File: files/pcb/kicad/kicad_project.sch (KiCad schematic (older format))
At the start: 19 parts, among them IC1 ATMEGA328-A, P1 CONN_6, SW1 SW_PUSH, U15 MY_PIN52, U16 MY_PIN52, U17 MY_PIN52, U18 MY_PIN52, X1 12MHz

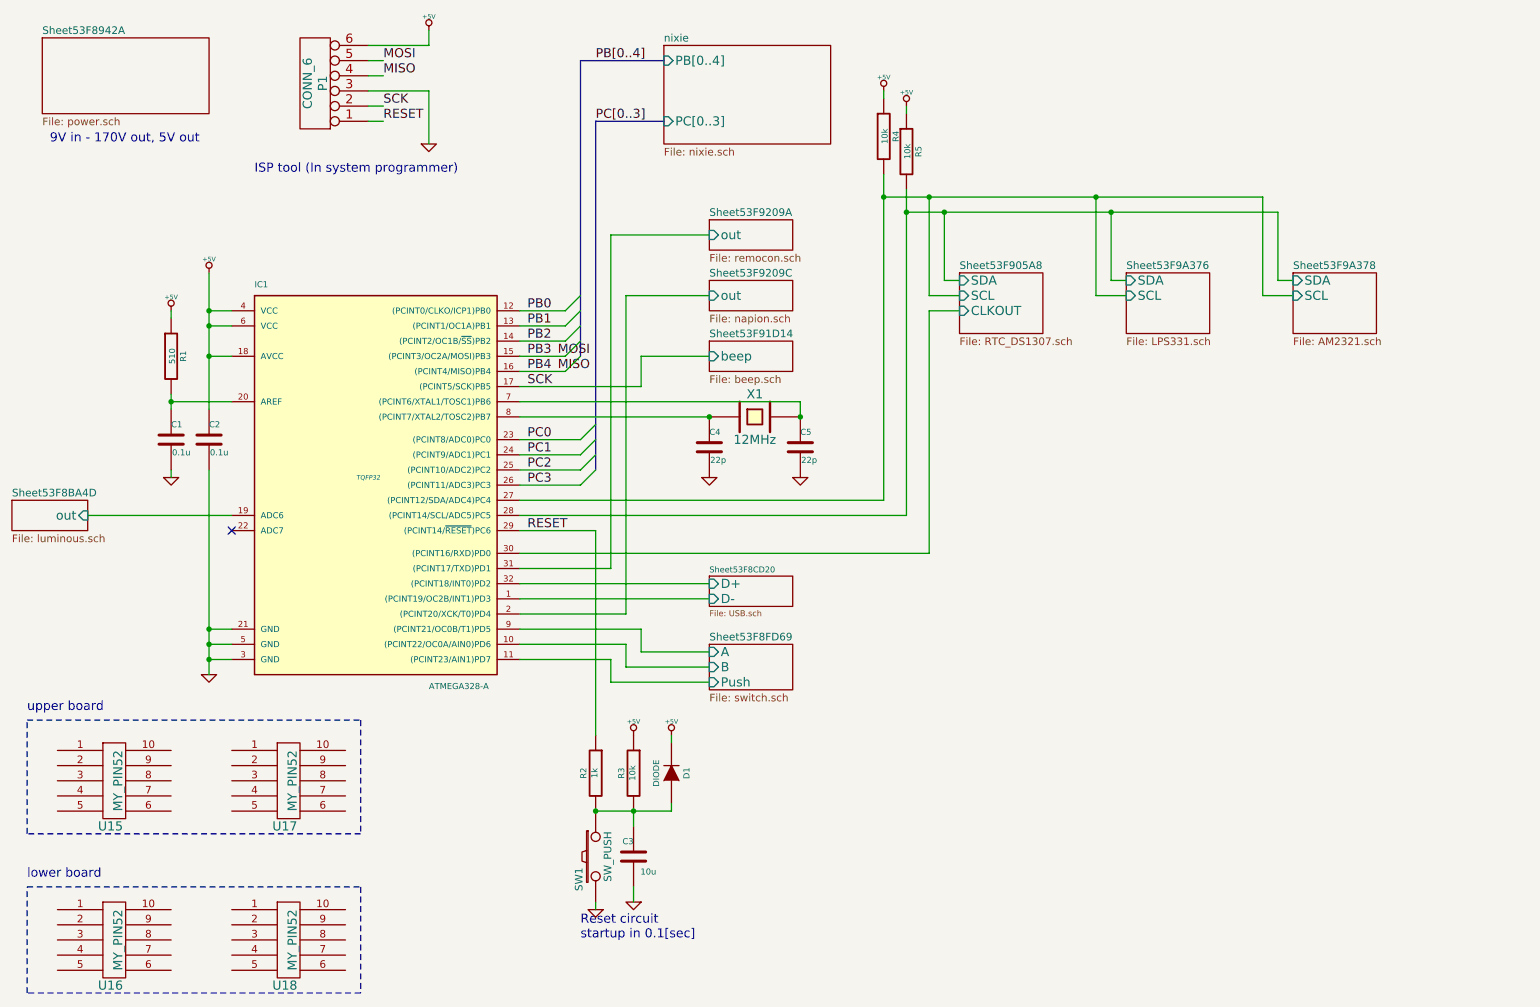
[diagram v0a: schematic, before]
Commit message: PCB
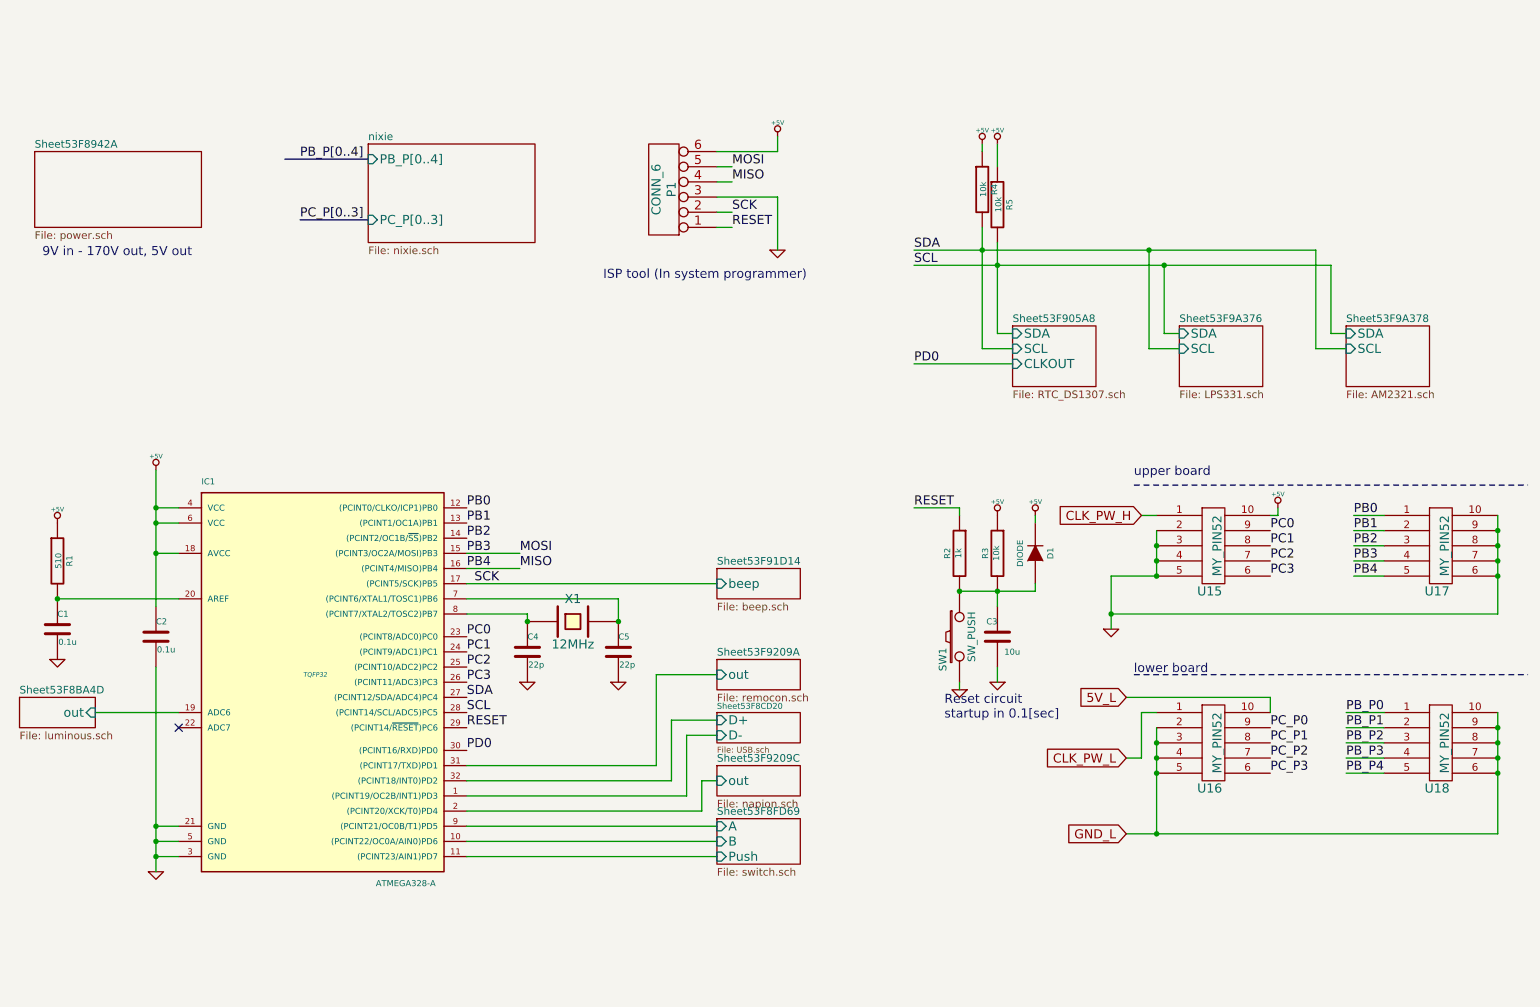
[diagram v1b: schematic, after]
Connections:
- net +5V: now also U15.10
- net GND: now also U15.2, U15.3, U15.4, U15.5, U17.10, U17.6, U17.7, U17.8, U17.9
- net MISO: now also U17.5
- net MOSI: now also U17.4
- net PB0: now also U17.1
- net PB1: now also U17.2
- net PB2: now also U17.3
- net PC0: now also U15.9
- net PC1: now also U15.8
- net PC2: now also U15.7
- net PC3: now also U15.6
- net CLK_PW_H: now reaches U15.1
- net PB_P0: now reaches U18.1
- net GND_L: now reaches U18.10
- net GND_L: now also U16.2, U16.3, U16.4, U16.5, U18.6, U18.7, U18.8, U18.9
- net PB_P1: now reaches U18.2
- net PB_P2: now reaches U18.3
- net PB_P3: now reaches U18.4
- net PB_P4: now reaches U18.5
- net CLK_PW_L: now reaches U16.1
- net 5V_L: now reaches U16.10
- net PC_P3: now reaches U16.6
- net PC_P2: now reaches U16.7
- net PC_P1: now reaches U16.8
- net PC_P0: now reaches U16.9
- net Sheet53F905A8/CLKOUT renamed PD0
- net Sheet53F905A8/SCL renamed SDA
- net Sheet53F905A8/SDA renamed SCL
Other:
- moved on the sheet: C1, C2, C3, C4, C5, D1, IC1, P1, R1, R2, R3, R4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
